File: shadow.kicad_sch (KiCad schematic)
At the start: 7 parts, among them SW1 SW_Push, SW2 SW_Push

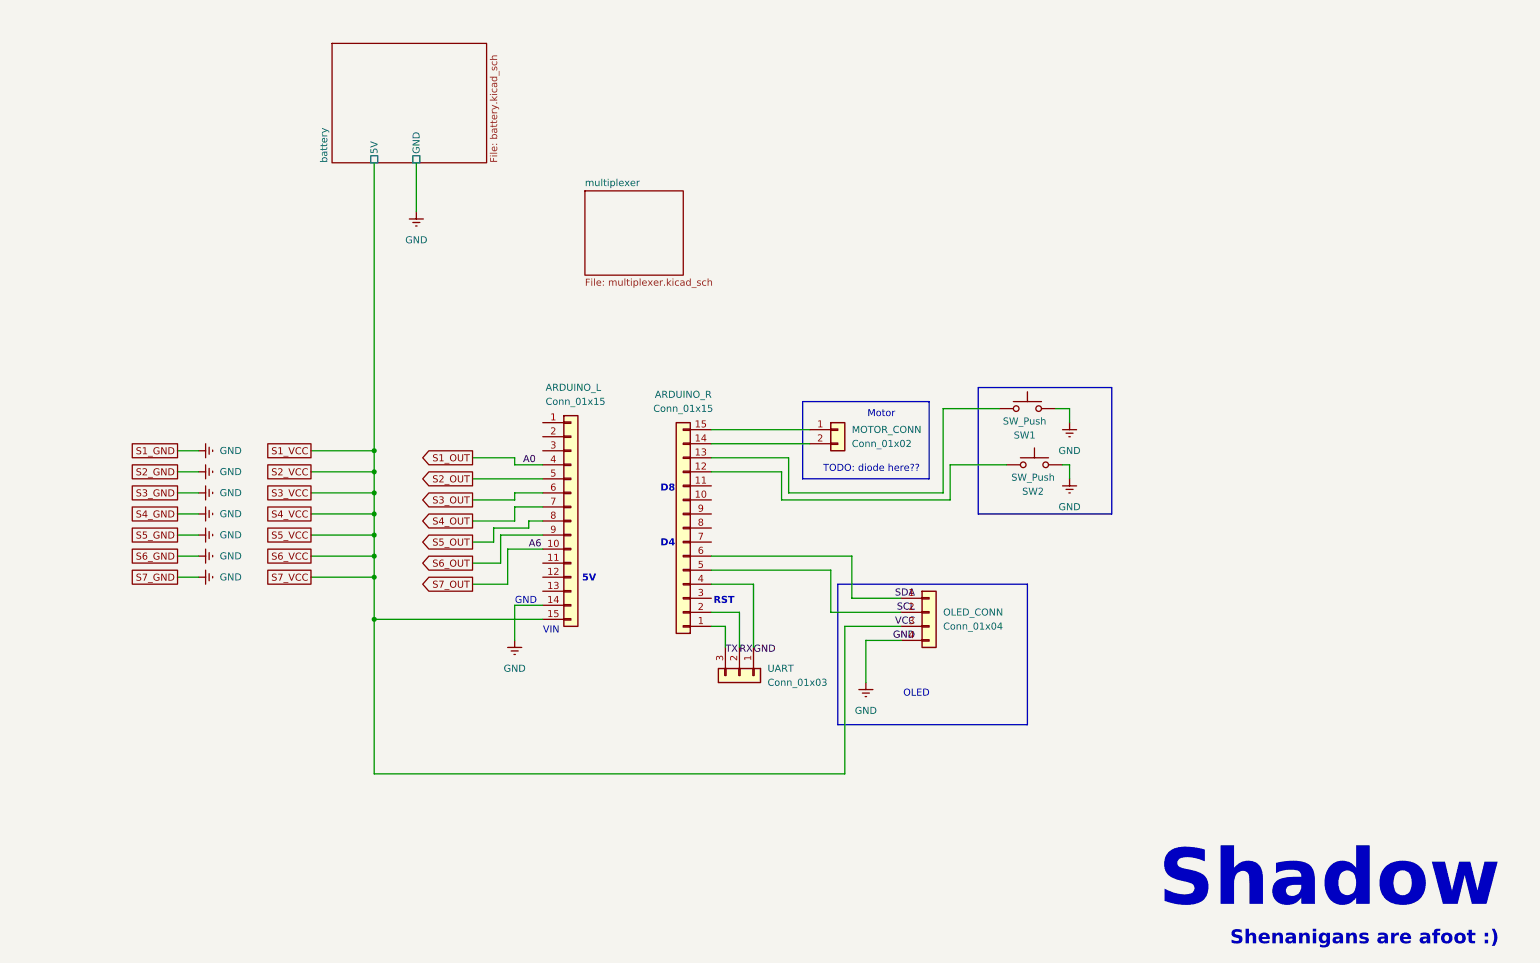
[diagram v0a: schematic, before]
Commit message: FINISH SCHEMATICS
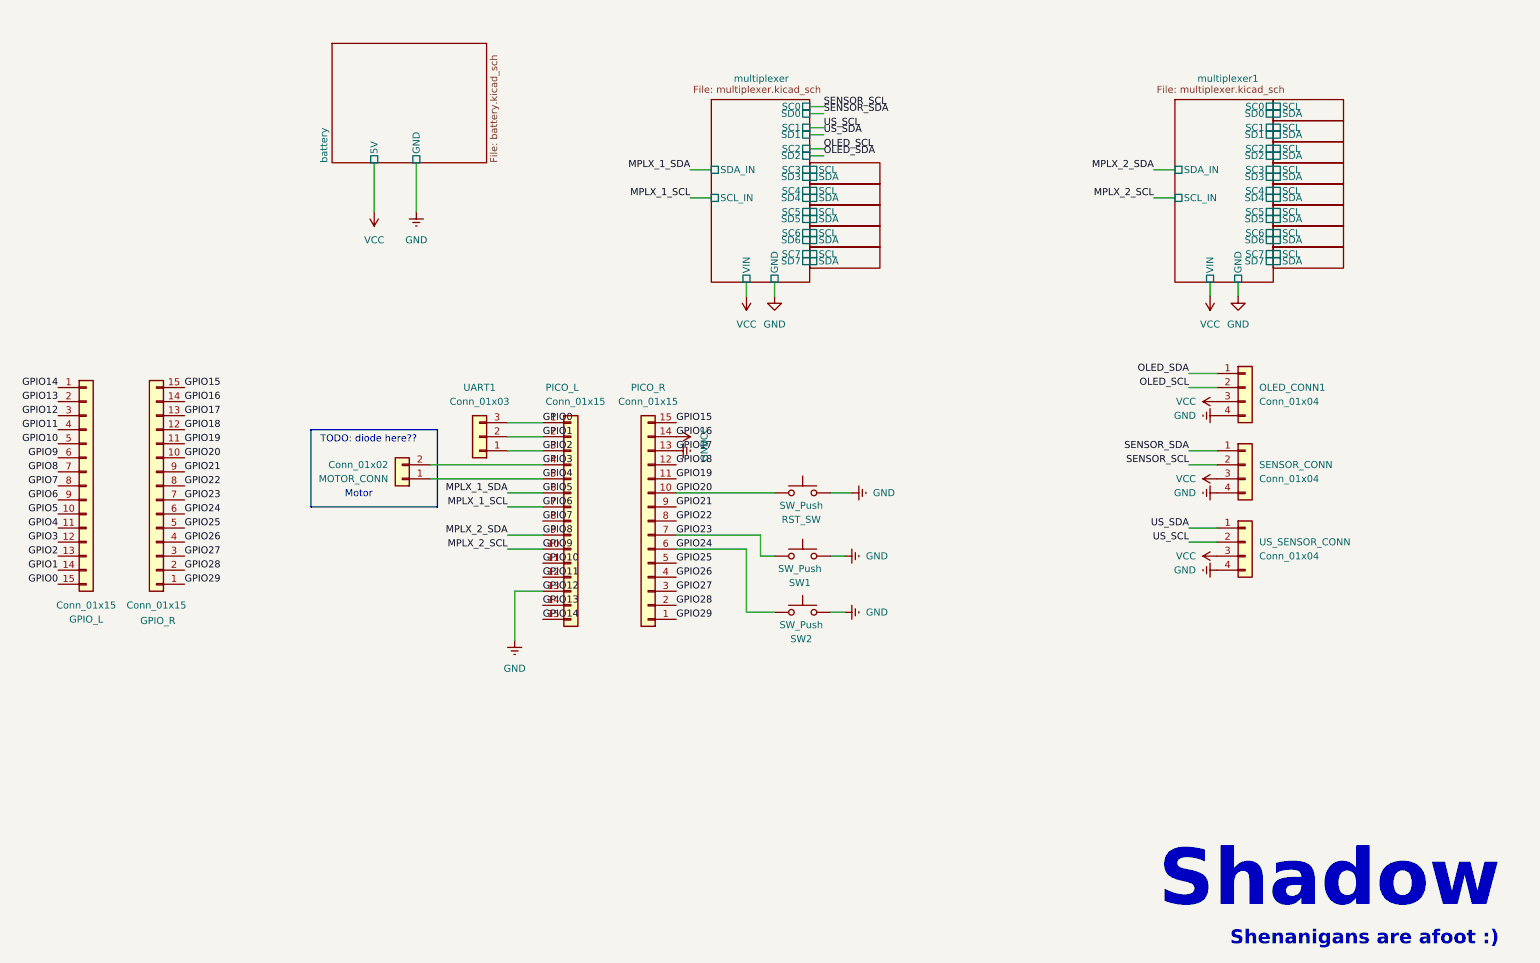
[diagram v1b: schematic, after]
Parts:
- removed OLED_CONN: Conn_01x04, symbol Connector_Generic:Conn_01x04
- removed UART: Conn_01x03, symbol Connector_Generic:Conn_01x03
- added GPIO_L, GPIO_R: Conn_01x15, symbol Connector_Generic:Conn_01x15
- added OLED_CONN1, SENSOR_CONN, US_SENSOR_CONN: Conn_01x04, symbol Connector_Generic:Conn_01x04
- added RST_SW: SW_Push, Button_Switch_THT:SW_PUSH-12mm, symbol Switch:SW_Push
- added UART1: Conn_01x03, symbol Connector_Generic:Conn_01x03
- renumbered ARDUINO_L to PICO_L, ARDUINO_R to PICO_R
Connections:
- net S1_OUT is gone; now on net GPIO3: PICO_L.4 (Pin_4)
- net GND: now also PICO_L.13 (Pin_13), PICO_R.13 (Pin_13), GPIO_L.3 (Pin_3), GPIO_R.13 (Pin_13), OLED_CONN1.4 (Pin_4), RST_SW.2, SENSOR_CONN.4 (Pin_4), US_SENSOR_CONN.4 (Pin_4); no longer PICO_L.14 (Pin_14)
- net VCC: now also PICO_R.14 (Pin_14), GPIO_R.14 (Pin_14), OLED_CONN1.3 (Pin_3), SENSOR_CONN.3 (Pin_3), US_SENSOR_CONN.3 (Pin_3)
- net GPIO15: now reaches PICO_R.15 (Pin_15)
- net GPIO15: now also GPIO_R.15 (Pin_15); no longer MOTOR_CONN.1 (Pin_1)
- net GPIO3: now reaches MOTOR_CONN.2 (Pin_2)
- net GPIO3: now also GPIO_L.12 (Pin_12); no longer PICO_R.14 (Pin_14)
- net GPIO18: now reaches PICO_R.12 (Pin_12)
- net GPIO18: now also GPIO_R.12 (Pin_12); no longer SW2.1
- net GPIO26: now reaches PICO_R.4 (Pin_4)
- net GPIO26: now also GPIO_R.4 (Pin_4)
- net GPIO28: now reaches PICO_R.2 (Pin_2)
- net GPIO28: now also GPIO_R.2 (Pin_2)
- net GPIO29: now reaches PICO_R.1 (Pin_1)
- net GPIO29: now also GPIO_R.1 (Pin_1)
- net GPIO24: now reaches PICO_R.6 (Pin_6)
- net GPIO24: now also SW2.1, GPIO_R.6 (Pin_6)
- net GPIO25: now reaches PICO_R.5 (Pin_5)
- net GPIO25: now also GPIO_R.5 (Pin_5)
- net GPIO20: now reaches PICO_R.10 (Pin_10)
- net GPIO20: now also GPIO_R.10 (Pin_10), RST_SW.1
- net GPIO19: now reaches PICO_R.11 (Pin_11)
- net GPIO19: now also GPIO_R.11 (Pin_11)
- net GPIO23: now reaches SW1.1
- net GPIO23: now also PICO_R.7 (Pin_7), GPIO_R.7 (Pin_7); no longer PICO_R.13 (Pin_13)
- net GPIO27: now reaches PICO_R.3 (Pin_3)
- net GPIO27: now also GPIO_R.3 (Pin_3)
- net GPIO22: now reaches PICO_R.8 (Pin_8)
- net GPIO22: now also GPIO_R.8 (Pin_8)
- net GPIO21: now reaches PICO_R.9 (Pin_9)
- net GPIO21: now also GPIO_R.9 (Pin_9)
- net GPIO0: now reaches PICO_L.1 (Pin_1)
- net GPIO0: now also GPIO_L.15 (Pin_15), UART1.3 (Pin_3)
- net GPIO10: now reaches PICO_L.11 (Pin_11)
- net GPIO10: now also GPIO_L.5 (Pin_5)
- net GPIO11: now reaches PICO_L.12 (Pin_12)
- net GPIO11: now also GPIO_L.4 (Pin_4)
- net GPIO1: now reaches PICO_L.2 (Pin_2)
- net GPIO1: now also GPIO_L.14 (Pin_14), UART1.2 (Pin_2)
- net GPIO2: now reaches PICO_L.3 (Pin_3)
- net GPIO2: now also GPIO_L.13 (Pin_13), UART1.1 (Pin_1)
- net S1_VCC renamed GPIO14
- net GPIO14: now also GPIO_L.1 (Pin_1)
- net S2_OUT renamed GPIO4
- net GPIO4: now also MOTOR_CONN.1 (Pin_1), GPIO_L.11 (Pin_11)
- net S3_OUT renamed GPIO5
- net GPIO5: now also GPIO_L.10 (Pin_10)
- net S4_OUT renamed GPIO6
- net GPIO6: now also GPIO_L.9 (Pin_9)
- net S5_OUT renamed GPIO7
- net GPIO7: now also GPIO_L.8 (Pin_8)
- net S6_OUT renamed GPIO8
- net GPIO8: now also GPIO_L.7 (Pin_7)
- net S7_OUT renamed GPIO9
- net GPIO9: now also GPIO_L.6 (Pin_6)
- new net GPIO13: GPIO_L.2 (Pin_2), PICO_L.14 (Pin_14)
- new net OLED_SCL: OLED_CONN1.2 (Pin_2)
- new net OLED_SDA: OLED_CONN1.1 (Pin_1)
- new net SENSOR_SCL: SENSOR_CONN.2 (Pin_2)
- new net SENSOR_SDA: SENSOR_CONN.1 (Pin_1)
- new net US_SCL: US_SENSOR_CONN.2 (Pin_2)
- new net US_SDA: US_SENSOR_CONN.1 (Pin_1)
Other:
- added sheet I2C_PINOUT (I2C_PINOUT.kicad_sch)
- added sheet I2C_PINOUT1 (I2C_PINOUT.kicad_sch)
- added sheet I2C_PINOUT10 (I2C_PINOUT.kicad_sch)
- added sheet I2C_PINOUT11 (I2C_PINOUT.kicad_sch)
- added sheet I2C_PINOUT12 (I2C_PINOUT.kicad_sch)
- added sheet I2C_PINOUT2 (I2C_PINOUT.kicad_sch)
- added sheet I2C_PINOUT3 (I2C_PINOUT.kicad_sch)
- added sheet I2C_PINOUT4 (I2C_PINOUT.kicad_sch)
- added sheet I2C_PINOUT5 (I2C_PINOUT.kicad_sch)
- added sheet I2C_PINOUT6 (I2C_PINOUT.kicad_sch)
- added sheet I2C_PINOUT7 (I2C_PINOUT.kicad_sch)
- added sheet I2C_PINOUT8 (I2C_PINOUT.kicad_sch)
- added sheet I2C_PINOUT9 (I2C_PINOUT.kicad_sch)
- added sheet multiplexer1 (multiplexer.kicad_sch)
- sheet multiplexer ports: added GND, SC0, SC1, SC2, SC3, SC4, SC5, SC6, SC7, SCL_IN, SD0, SD1, SD2, SD3, SD4, SD5, SD6, SD7, SDA_IN, VIN; removed none
- note removed: "5V"
- note removed: "D4"
- note removed: "D8"
- note removed: "GND"
- note removed: "OLED"
- note removed: "RST"
- note removed: "VIN"
- moved on the sheet: MOTOR_CONN, PICO_R, SW1, SW2
